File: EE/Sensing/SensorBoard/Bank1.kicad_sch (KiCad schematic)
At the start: 35 parts

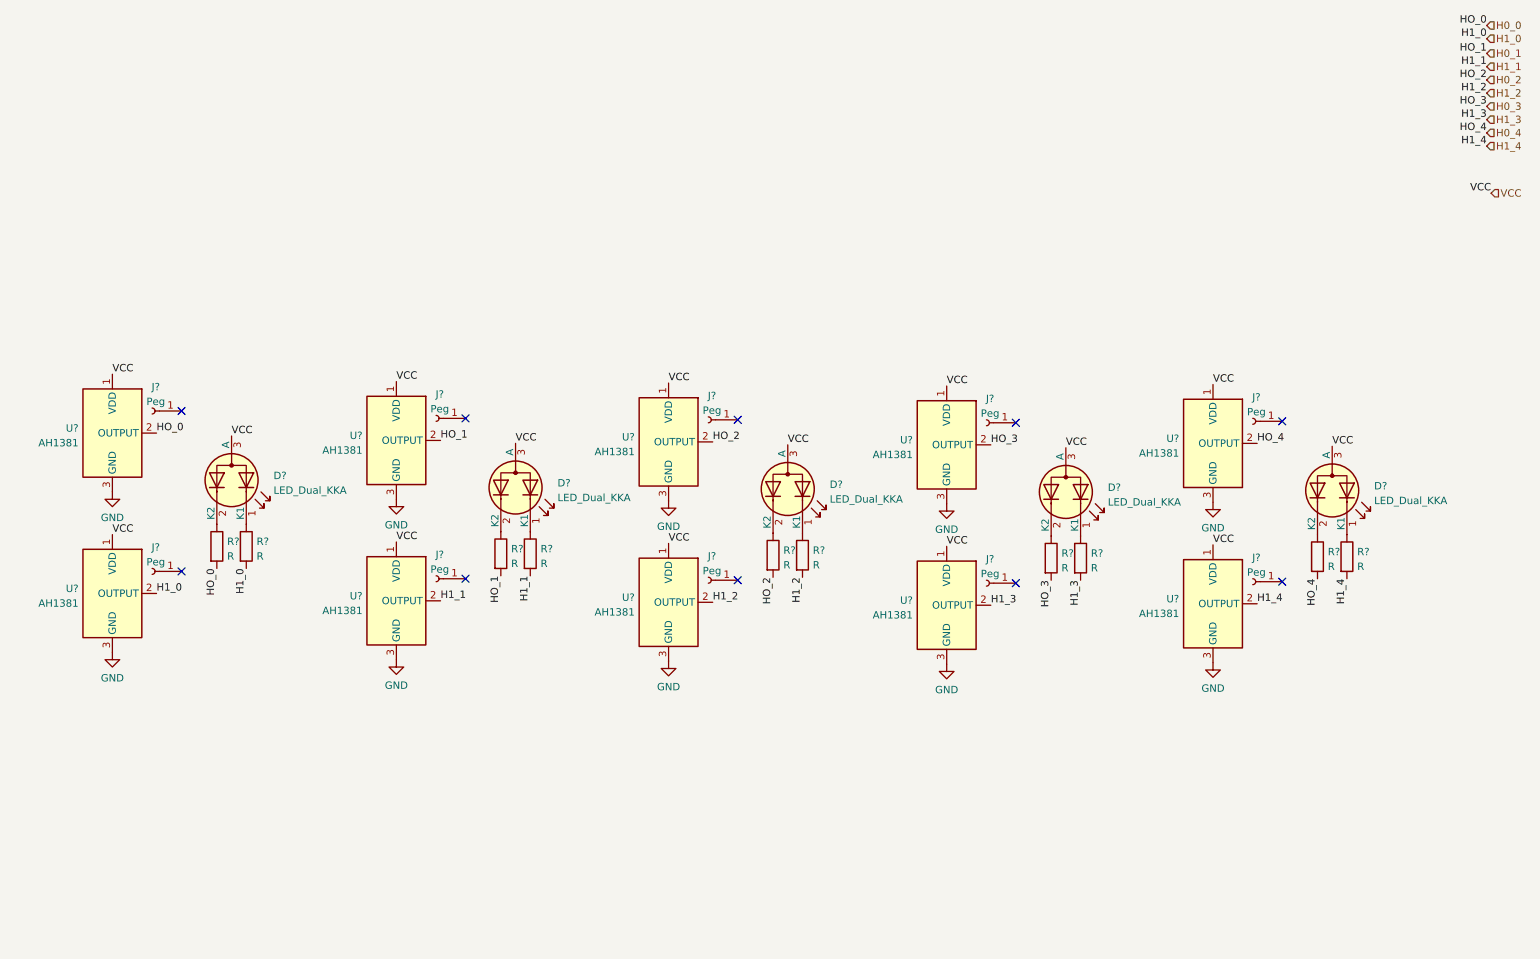
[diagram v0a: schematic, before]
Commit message: WIP - TBs ordered, Sensor board pre layout sensor board
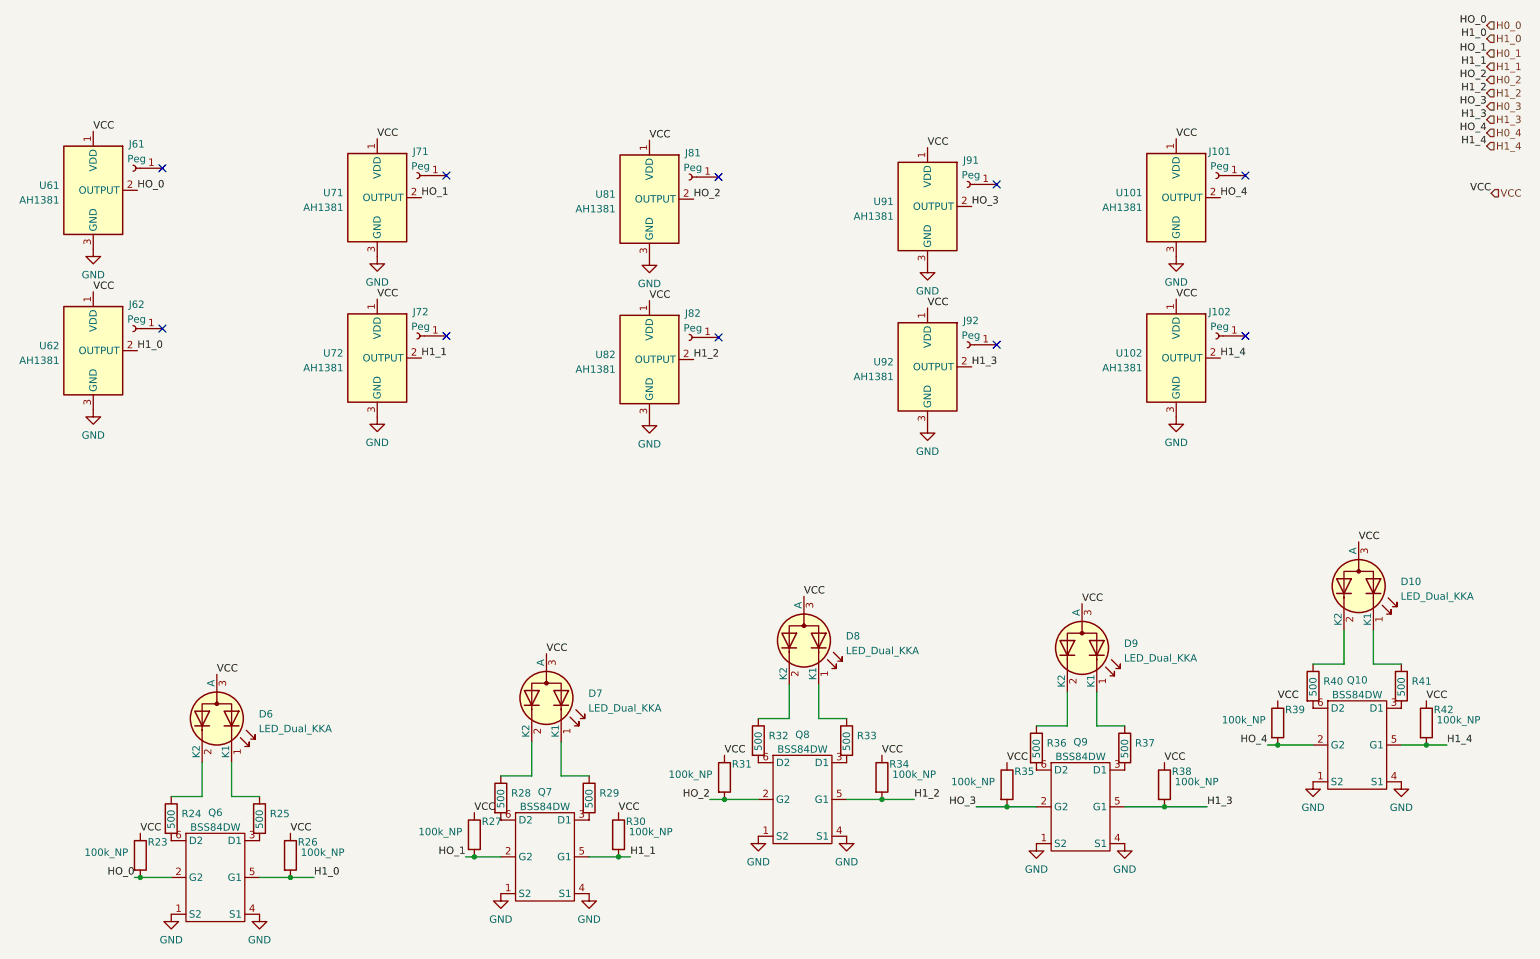
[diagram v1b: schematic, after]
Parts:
- removed D? (x5): LED_Dual_KKA, symbol Device:LED_Dual_KKA
- removed J? (x10): Peg, symbol Connector:Conn_01x01_Female
- removed R? (x10): R, Resistor_SMD:R_0402_1005Metric_Pad0.72x0.64mm_HandSolder, symbol Device:R
- removed U? (x10): AH1381, Package_TO_SOT_SMD:SOT-23, symbol Sensor_Magnetic:AH1806-W
- added D10, D6, D7, D8, D9: LED_Dual_KKA, Package_TO_SOT_SMD:SC-59, symbol Device:LED_Dual_KKA
- added J101, J102, J61, J62, J71, J72, J81, J82, J91, J92: Peg, Library:TestPattern0, symbol Connector:Conn_01x01_Female
- added Q10, Q6, Q7, Q8, Q9: BSS84DW, Package_TO_SOT_SMD:SOT-363_SC-70-6, symbol New_Library:BSS84DW
- added R23, R26, R27, R30, R31, R34, R35, R38, R39, R42: 100k_NP, Resistor_SMD:R_0402_1005Metric_Pad0.72x0.64mm_HandSolder, symbol Device:R
- added R24, R25, R28, R29, R32, R33, R36, R37, R40, R41: 500, Resistor_SMD:R_0402_1005Metric_Pad0.72x0.64mm_HandSolder, symbol Device:R
- added U101, U102, U61, U62, U71, U72, U81, U82, U91, U92: AH1381, Package_TO_SOT_SMD:SOT-23, symbol Sensor_Magnetic:AH1806-W
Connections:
- net GND: now also Q10.1 (S2), Q10.4 (S1), Q6.1 (S2), Q6.4 (S1), Q7.1 (S2), Q7.4 (S1), Q8.1 (S2), Q8.4 (S1), Q9.1 (S2), Q9.4 (S1), U101.3 (GND), U102.3 (GND), U61.3 (GND), U62.3 (GND), U71.3 (GND), U72.3 (GND), U81.3 (GND), U82.3 (GND), U91.3 (GND), U92.3 (GND)
- net H0_0: now also Q6.2 (G2), R23.2, U61.2 (OUTPUT)
- net H0_1: now also Q7.2 (G2), R27.2, U71.2 (OUTPUT)
- net H0_2: now also Q8.2 (G2), R31.2, U81.2 (OUTPUT)
- net H0_3: now also Q9.2 (G2), R35.2, U91.2 (OUTPUT)
- net H0_4: now also Q10.2 (G2), R39.2, U101.2 (OUTPUT)
- net H1_0: now also Q6.5 (G1), R26.2, U62.2 (OUTPUT)
- net H1_1: now also Q7.5 (G1), R30.2, U72.2 (OUTPUT)
- net H1_2: now also Q8.5 (G1), R34.2, U82.2 (OUTPUT)
- net H1_3: now also Q9.5 (G1), R38.2, U92.2 (OUTPUT)
- net H1_4: now also Q10.5 (G1), R42.2, U102.2 (OUTPUT)
- net VCC: now also D10.3 (A), D6.3 (A), D7.3 (A), D8.3 (A), D9.3 (A), R23.1, R26.1, R27.1, R30.1, R31.1, R34.1, R35.1, R38.1, R39.1, R42.1, U101.1 (VDD), U102.1 (VDD), U61.1 (VDD), U62.1 (VDD), U71.1 (VDD), U72.1 (VDD), U81.1 (VDD), U82.1 (VDD), U91.1 (VDD), U92.1 (VDD)
- new net: D7.1 (K1), R29.1
- new net: D7.2 (K2), R28.1
- new net: D10.1 (K1), R41.1
- new net: Q10.3 (D1), R41.2
- new net: D8.1 (K1), R33.1
- new net: D8.2 (K2), R32.1
- new net: D9.2 (K2), R36.1
- new net: Q9.6 (D2), R36.2
- new net: Q7.6 (D2), R28.2
- new net: Q8.6 (D2), R32.2
- new net: D9.1 (K1), R37.1
- new net: Q9.3 (D1), R37.2
- new net: Q7.3 (D1), R29.2
- new net: Q10.6 (D2), R40.2
- new net: D6.2 (K2), R24.1
- new net: Q6.6 (D2), R24.2
- new net: D10.2 (K2), R40.1
- new net: D6.1 (K1), R25.1
- new net: Q6.3 (D1), R25.2
- new net: Q8.3 (D1), R33.2
